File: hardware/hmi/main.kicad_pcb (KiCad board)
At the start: 2 copper layers, 80 x 80 mm, 54 parts, among them J1 LOAD_CON, J2 Conn_01x08, J3 SD_CARD, J4 ENCODER, SW1 CC, SW2 CV, SW3 CR, SW4 CP, SW5 EN, U1 ESP32-DEVKIT-V1

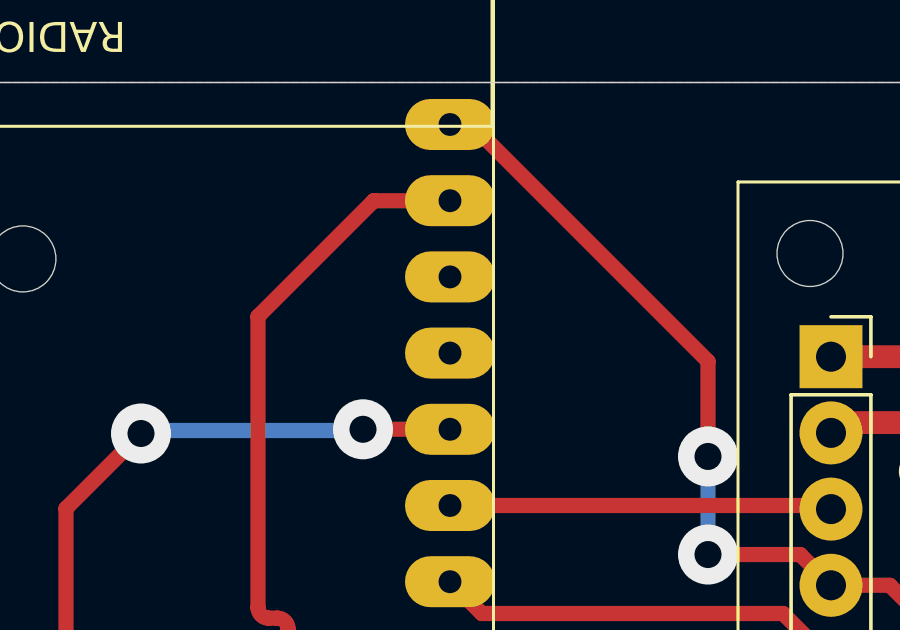
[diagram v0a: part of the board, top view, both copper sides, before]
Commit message: WIP hardware
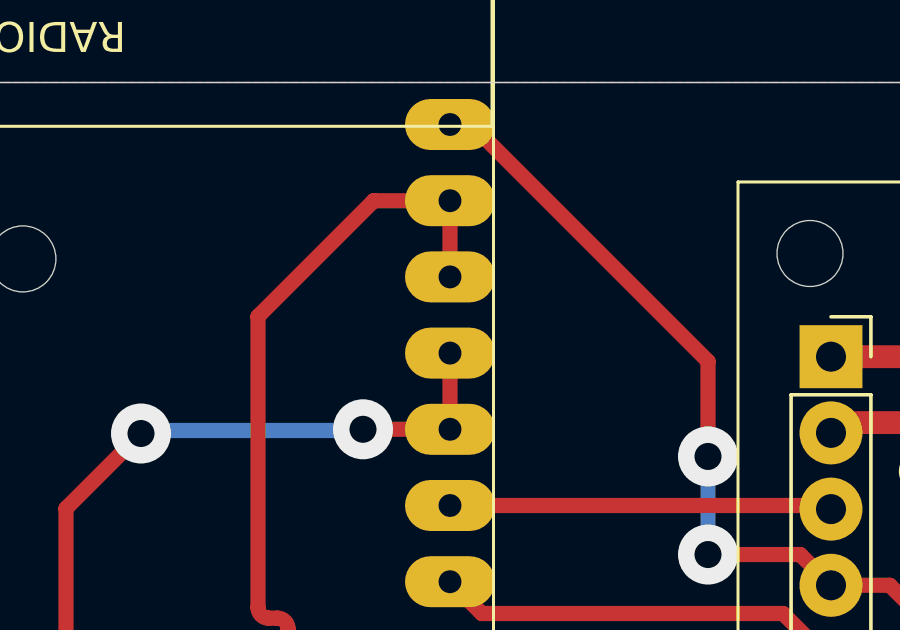
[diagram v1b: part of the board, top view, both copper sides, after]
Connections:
- U1 pad 12: unconnected-(U1-GPIO_3/RX0-Pad12) -> /LOAD_SCL
- U1 pad 13: unconnected-(U1-GPIO_1/TX0-Pad13) -> /LOAD_SDA
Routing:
- net /LOAD_SDA: track 65.0 -> 67.5 mm
- net /LOAD_SCL: track 64.0 -> 66.5 mm
